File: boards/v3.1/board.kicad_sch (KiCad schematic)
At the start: 65 parts, among them J1 KF301-2P, J2 KF301-2P, J3 KF301-2P, J4 KF301-2P, J5 KF301-2P, J6 KF301-2P, P1 Pin Header, P2 Pin Header, P3 Pin Header, P4 Pin Header, P5 Pin Header, SW1 SS-12D00G 4mm, SW2 SS-12D00G 4mm, T1 ZMPT101B, T2 ZMPT101B, T3 ZMPT101B, U1 TL082, U2 TL082, U3 TL082, U4 TL082, U5 TL082, U6 TL082

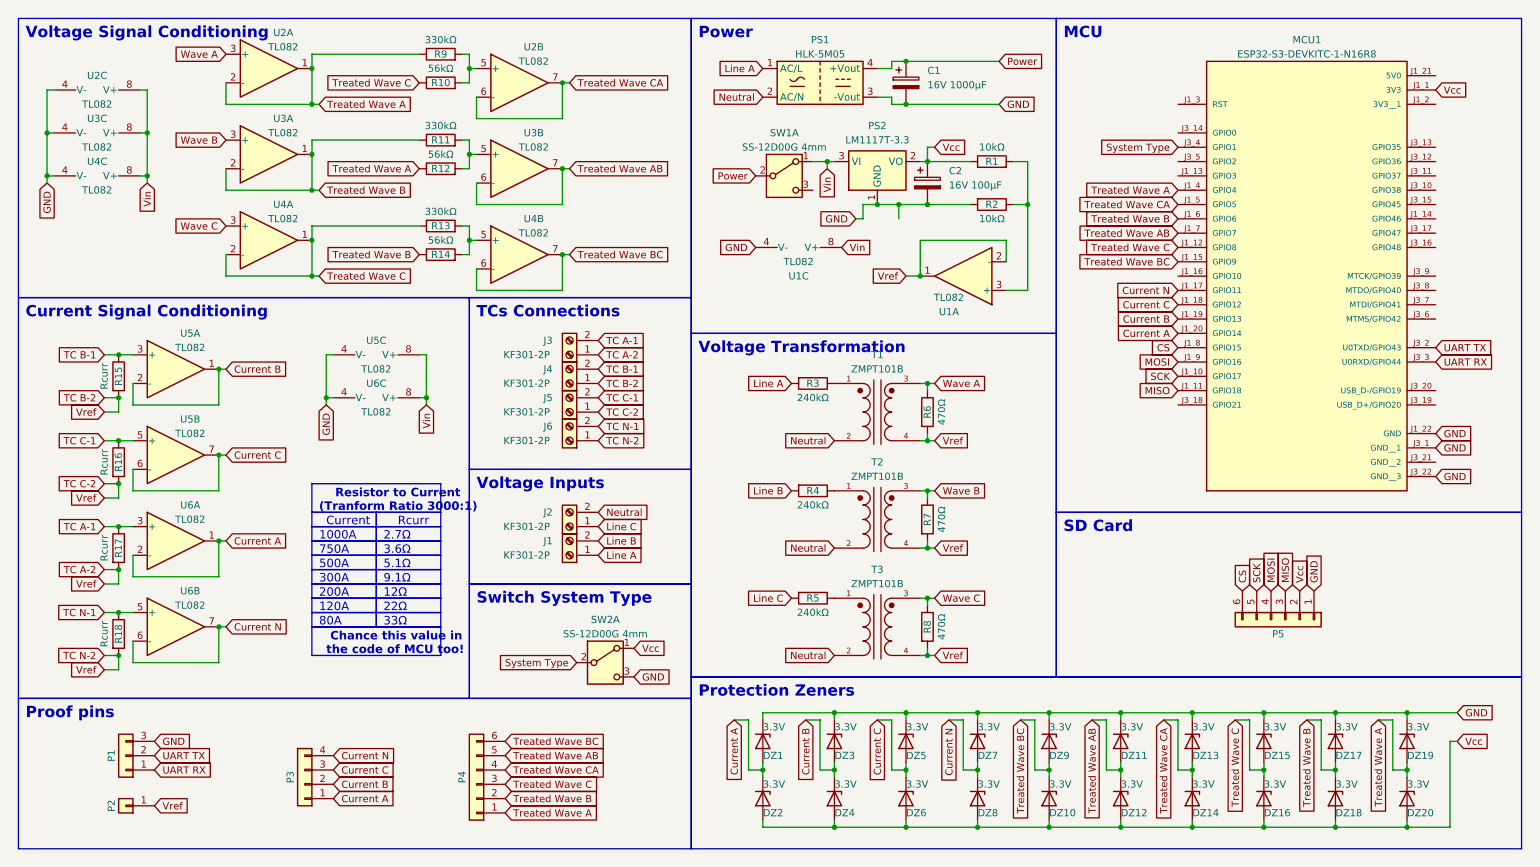
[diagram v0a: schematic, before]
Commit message: Update firmware and boards
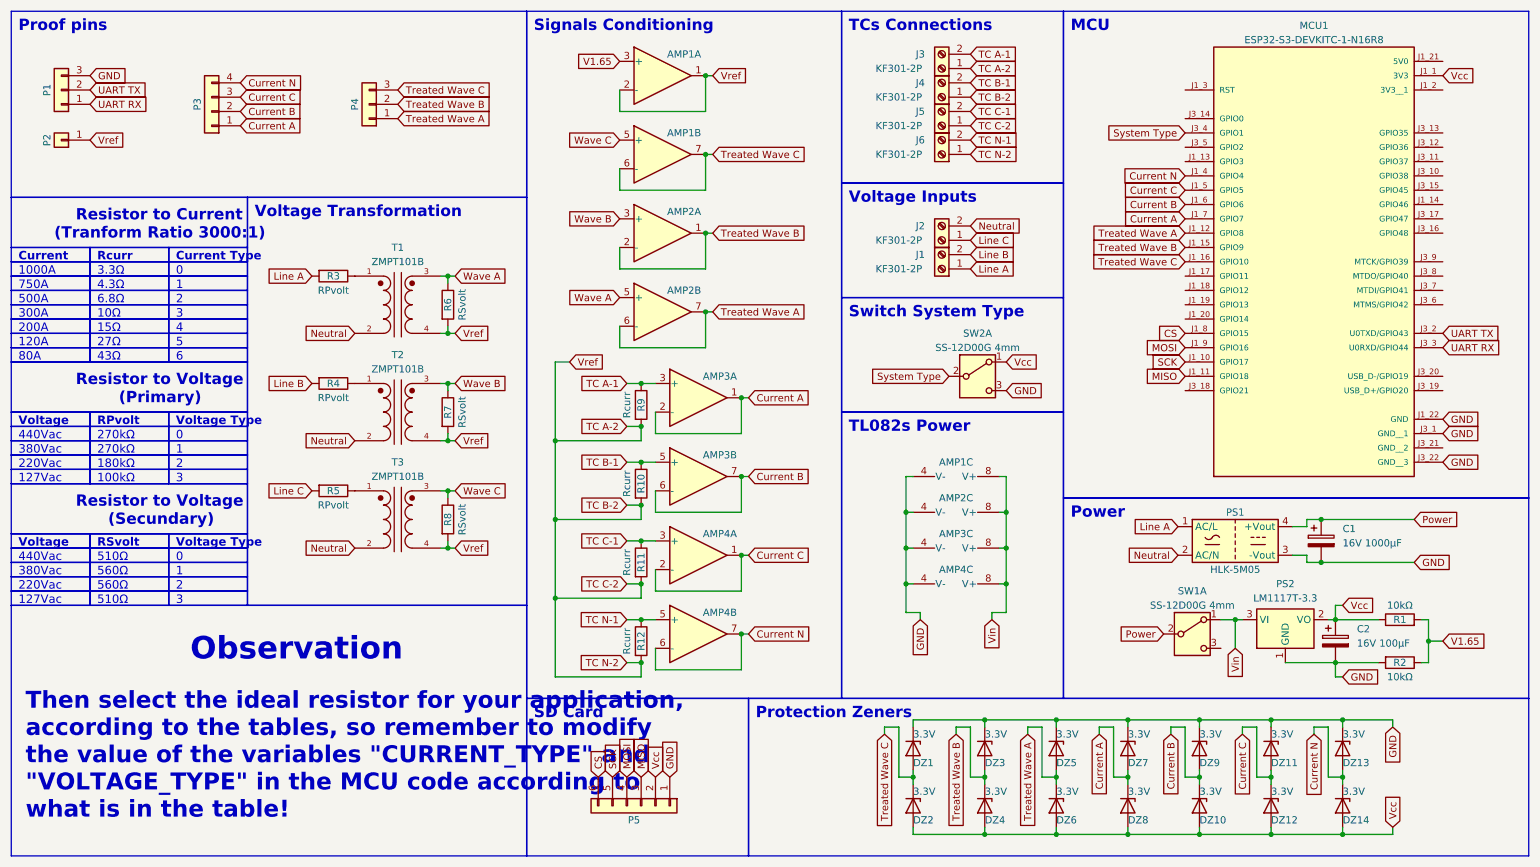
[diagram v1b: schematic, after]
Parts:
- removed DZ15, DZ16, DZ17, DZ18, DZ19, DZ20: 3.3V, Diode_THT:D_DO-34_SOD68_P7.62mm_Horizontal, symbol Device:D_Zener
- removed P4: Pin Header, Connector_PinHeader_2.54mm:PinHeader_1x06_P2.54mm_Vertical, symbol Connector_Generic:Conn_01x06
- removed R10, R12, R14: 56kΩ, Resistor_THT:R_Axial_DIN0207_L6.3mm_D2.5mm_P10.16mm_Horizontal, symbol Device:R
- removed R11, R13, R9: 330kΩ, Resistor_THT:R_Axial_DIN0207_L6.3mm_D2.5mm_P10.16mm_Horizontal, symbol Device:R
- removed unit 1 of U1
- removed U2, U3, U4, U5, U6: TL082, Package_DIP:DIP-8_W7.62mm_Socket, symbol Amplifier_Operational:TL082
- added unit 1 of AMP1
- added unit 2 of AMP1
- added AMP2, AMP3, AMP4: TL082, Package_DIP:DIP-8_W7.62mm_Socket, symbol Amplifier_Operational:TL082
- added P4: Pin Header, Connector_PinHeader_2.54mm:PinHeader_1x03_P2.54mm_Vertical, symbol Connector_Generic:Conn_01x03
- R3, R4, R5: value 240kΩ -> RPvolt
- R6, R7, R8: value 470Ω -> RSvolt
- renumbered U1 to AMP1, R16 to R10, R17 to R11, R18 to R12, R15 to R9
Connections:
- net Current A: now also DZ7.2 (A), DZ8.1 (K), MCU1.J1_7 (GPIO7), AMP3.1, AMP3.2 (-); no longer DZ1.2 (A), DZ2.1 (K), MCU1.J1_20 (GPIO14)
- net Current B: now also DZ10.1 (K), DZ9.2 (A), MCU1.J1_6 (GPIO6), AMP3.6 (-), AMP3.7; no longer DZ3.2 (A), DZ4.1 (K), MCU1.J1_19 (GPIO13)
- net Current C: now also DZ11.2 (A), DZ12.1 (K), MCU1.J1_5 (GPIO5), AMP4.1, AMP4.2 (-); no longer DZ5.2 (A), DZ6.1 (K), MCU1.J1_18 (GPIO12)
- net Current N: now also DZ13.2 (A), DZ14.1 (K), MCU1.J1_4 (GPIO4), AMP4.6 (-), AMP4.7; no longer DZ7.2 (A), DZ8.1 (K), MCU1.J1_17 (GPIO11)
- net GND: now also AMP2.4 (V-), AMP3.4 (V-), AMP4.4 (V-)
- net TC A-1: now also R9.1, AMP3.3 (+); no longer R11.1
- net TC A-2: now also AMP1.1, AMP1.2 (-)
- net TC B-1: now also R10.1, AMP3.5 (+); no longer R9.1
- net TC C-1: now also R11.1, AMP4.3 (+); no longer R10.1
- net TC N-1: now also AMP4.5 (+)
- net Treated Wave A: now also DZ5.2 (A), DZ6.1 (K), MCU1.J1_12 (GPIO8), AMP2.6 (-), AMP2.7, P4.1 (Pin_1); no longer MCU1.J1_4 (GPIO4)
- net Treated Wave B: now also DZ3.2 (A), DZ4.1 (K), MCU1.J1_15 (GPIO9), AMP2.1, AMP2.2 (-), P4.2 (Pin_2); no longer MCU1.J1_6 (GPIO6)
- net Treated Wave C: now also DZ1.2 (A), DZ2.1 (K), MCU1.J1_16 (GPIO10), AMP1.6 (-), AMP1.7, P4.3 (Pin_3); no longer MCU1.J1_12 (GPIO8)
- net Vin: now also AMP2.8 (V+), AMP3.8 (V+), AMP4.8 (V+)
- net Wave A: now also AMP2.5 (+)
- net Wave B: now also AMP2.3 (+)
- net Wave C: now also AMP1.5 (+)
- net V1.65: now reaches R1.2, R2.1
- net V1.65: now also AMP1.3 (+)
- removed net Treated Wave AB: DZ11.2 (A), DZ12.1 (K), MCU1.J1_7 (GPIO7)
- removed net Treated Wave BC: DZ10.1 (K), DZ9.2 (A), MCU1.J1_15 (GPIO9)
- removed net Treated Wave CA: DZ13.2 (A), DZ14.1 (K), MCU1.J1_5 (GPIO5)
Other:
- note added: "0"
- note added: "1"
- note added: "100kΩ"
- note added: "10Ω"
- note added: "127Vac"
- note added: "15Ω"
- note added: "180kΩ"
- note added: "2"
- note added: "220Vac"
- note added: "270kΩ"
- note added: "27Ω"
- note added: "3"
- note added: "3.3Ω"
- note added: "380Vac"
- note added: "4"
- note added: "4.3Ω"
- note added: "43Ω"
- note added: "440Vac"
- note added: "5"
- note added: "510Ω"
- note added: "560Ω"
- note added: "6"
- note added: "6.8Ω"
- note added: "Current Type"
- note added: "Observation"
- note added: "RPvolt"
- note added: "RSvolt"
- note added: "Resistor to Voltage (Primary)"
- note added: "Resistor to Voltage (Secundary)"
- note added: "Signals Conditioning"
- note added: "TL082s Power"
- note added: "Then select the ideal resistor for your application, according to the tables, so remember to modify the value of the variables "CURRENT_TYPE" and "VOLTAGE_TYPE" in the MCU code according to what is in the table!"
- note added: "Voltage"
- note added: "Voltage Type"
- note removed: "12Ω"
- note removed: "2.7Ω"
- note removed: "22Ω"
- note removed: "3.6Ω"
- note removed: "33Ω"
- note removed: "5.1Ω"
- note removed: "9.1Ω"
- note removed: "Chance this value in the code of MCU too!"
- note removed: "Current Signal Conditioning"
- note removed: "Voltage Signal Conditioning"
- title: ESP32 Power Analyser V3.0 Schematics -> ESP32 Power Analyser V4.0 Schematics
- moved on the sheet: AMP1C, C1, C2, DZ1, DZ10, DZ11, DZ12, DZ13, DZ14, DZ2, DZ3, DZ4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
